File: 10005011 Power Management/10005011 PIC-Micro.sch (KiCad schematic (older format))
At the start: 41 parts, among them IC1 LM393D, IC3 PIC18F6622, IC5 DS2480B, J2 ICSP, T2 IRLML5103

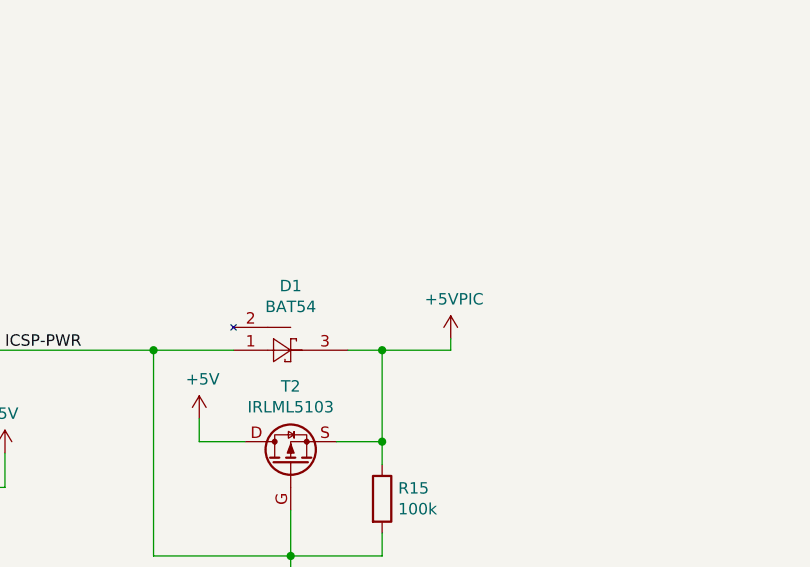
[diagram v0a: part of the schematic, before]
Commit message: Powermanagement dev, ERC
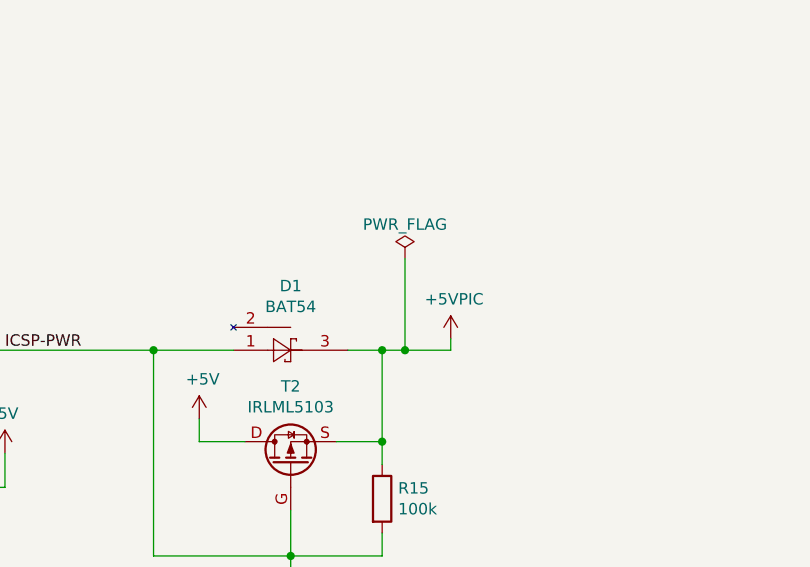
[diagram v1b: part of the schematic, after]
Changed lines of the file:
@@
 	6700 4750 7300 4750
 Wire Wire Line
-	4400 9500 4700 9500
+	4400 9500 4500 9500
 Wire Wire Line
 	3400 9500 3400 10400
@@
 Wire Wire Line
 	4700 9450 4700 9500
+$Comp
+L power:PWR_FLAG #FLG0116
+U 1 1 5ED8EE51
+P 4500 9100
+F 0 "#FLG0116" H 4500 9175 50  0001 C CNN
+F 1 "PWR_FLAG" H 4500 9250 50  0000 C CNN
+F 2 "" H 4500 9100 50  0001 C CNN
+F 3 "~" H 4500 9100 50  0001 C CNN
+	1    4500 9100
+	1    0    0    -1
+$EndComp
+Wire Wire Line
+	4500 9100 4500 9500
+Connection ~ 4500 9500
+Wire Wire Line
+	4500 9500 4700 9500
 $EndSCHEMATC
